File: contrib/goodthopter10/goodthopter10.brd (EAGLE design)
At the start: 210.2 x 143.8 mm, 24 parts, among them IC1 F22X4---DA38, IC2 FT232RL-BASICSSOP, Q2 20MHz

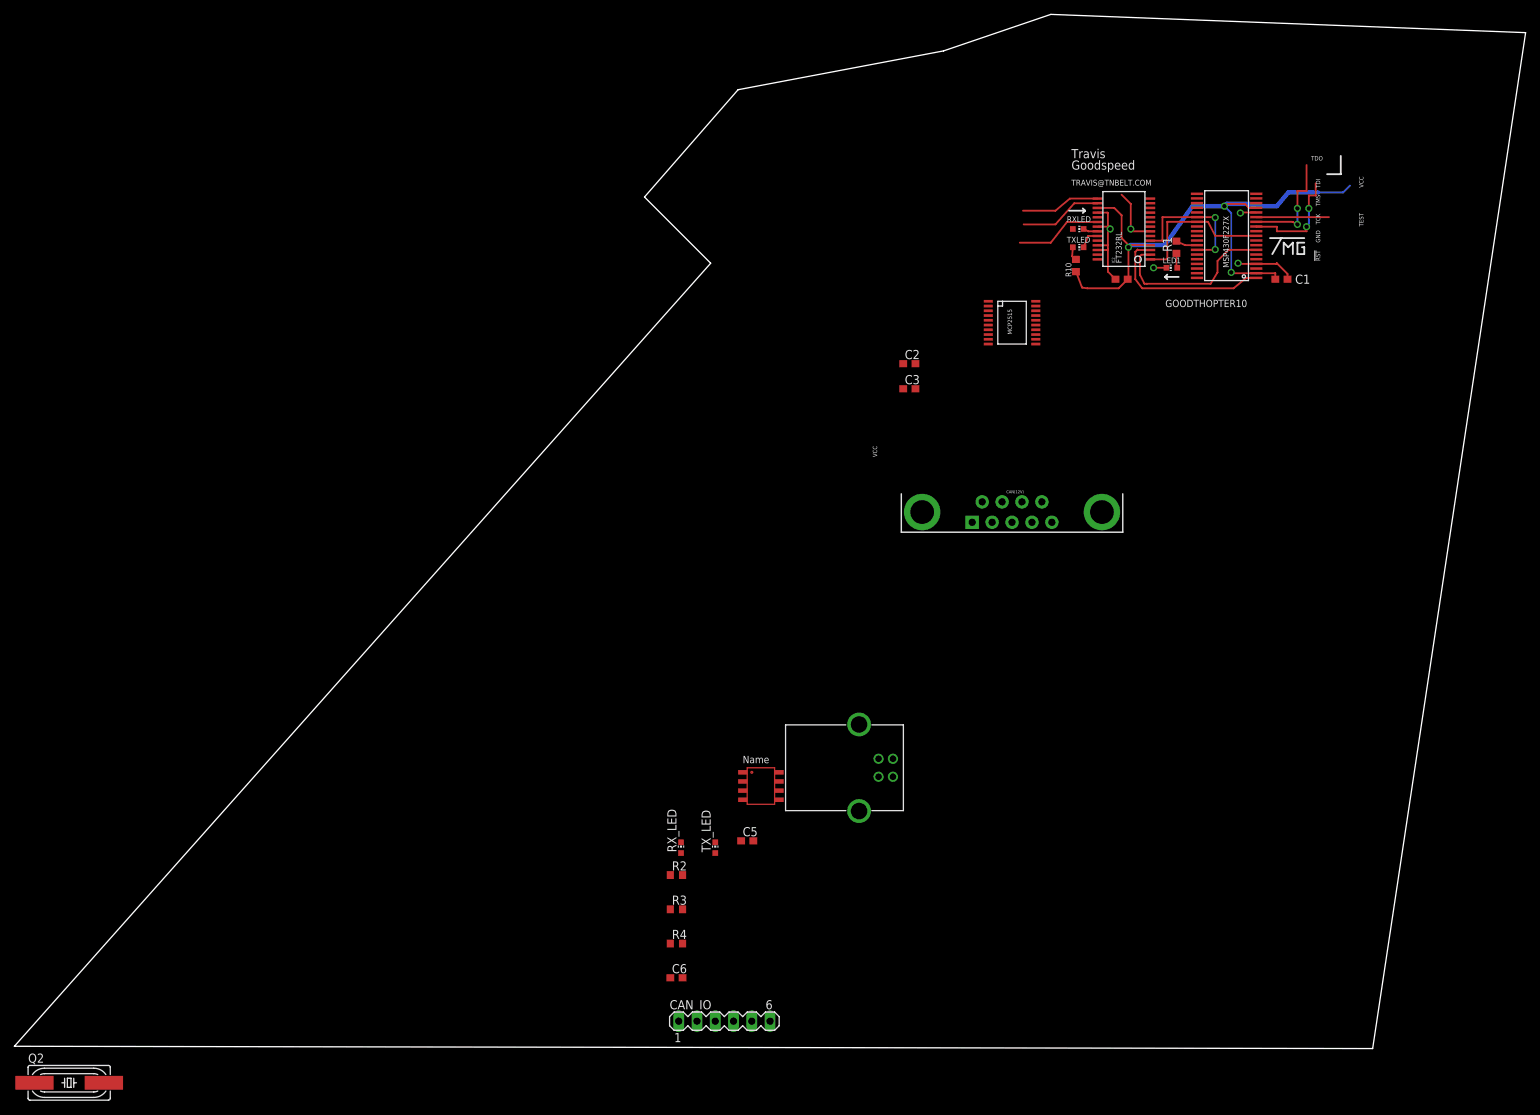
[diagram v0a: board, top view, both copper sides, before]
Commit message: Routing goodthopter10.brd, updated.
git-svn-id: https://svn.code.sf.net/p/goodfet/code@1213 12e2690d-a6be-4b82-a7b7-67c4a43b65c8
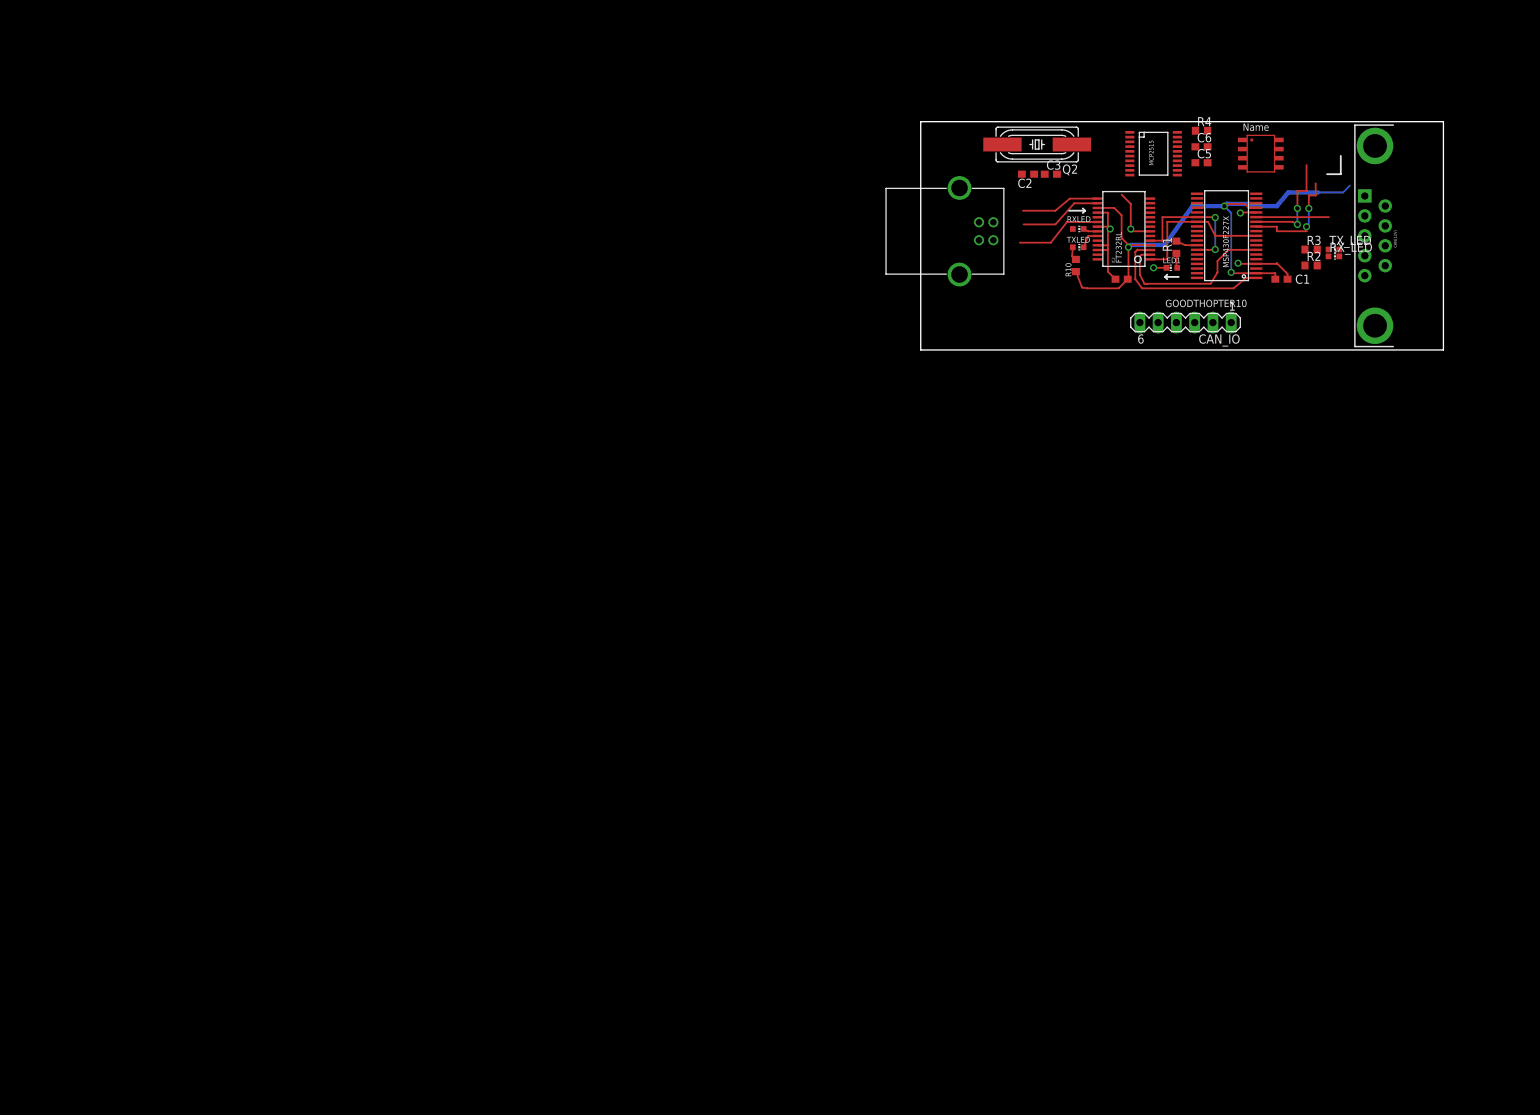
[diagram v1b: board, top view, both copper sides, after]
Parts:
- moved Q2 187.5 mm to (7.62, 21.6), turned to 180 degrees
- moved C6 136.7 mm to (30.5, 21.3)
- moved R4 134.6 mm to (30.5, 23.5)
- moved R3 127.3 mm to (45.7, 6.99)
- moved RX_LED 122.5 mm to (48.9, 6.03), turned to 270 degrees
- moved R2 122.4 mm to (45.7, 4.76)
- moved TX_LED 119.7 mm to (48.9, 6.99), turned to 270 degrees
- moved CAN_IO 116.4 mm to (28.3, -3.17), turned to 180 degrees
- moved C5 113.5 mm to (30.5, 19.1)
- moved U$2 112.1 mm to (38.7, 20.3)
- moved 292304-2 75.9 mm to (-3.17, 9.53)
- moved CAN(12V) 63.4 mm to (54.6, 8.89), turned to 270 degrees
- moved C3 35.8 mm to (9.53, 17.5)
- moved C2 31.1 mm to (6.35, 17.5), turned to 180 degrees
- moved U$1 30.7 mm to (23.8, 20.6)
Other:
- board size 210.2 x 143.8 mm -> 72.7 x 31.8 mm
- board text removed: "!RST"
- board text removed: "GND"
- board text removed: "Goodspeed"
- board text removed: "TCK"
- board text removed: "TDI"
- board text removed: "TDO"
- board text removed: "TEST"
- board text removed: "TMS"
- board text removed: "TRAVIS@TNBELT.COM"
- board text removed: "Travis"
- board text removed: "VCC"

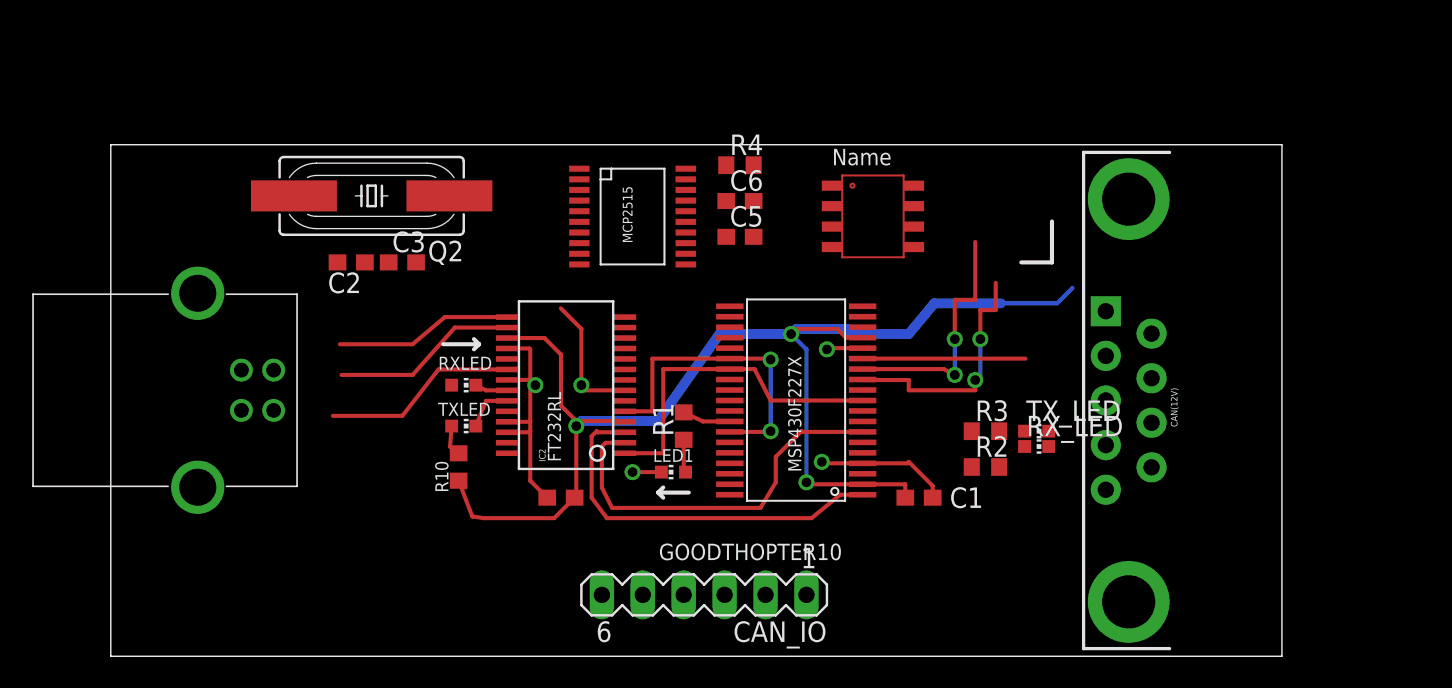
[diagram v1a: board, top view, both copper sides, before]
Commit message: Completed GoodThopter10 Routing, Gerbers Added, README.
git-svn-id: https://svn.code.sf.net/p/goodfet/code@1214 12e2690d-a6be-4b82-a7b7-67c4a43b65c8
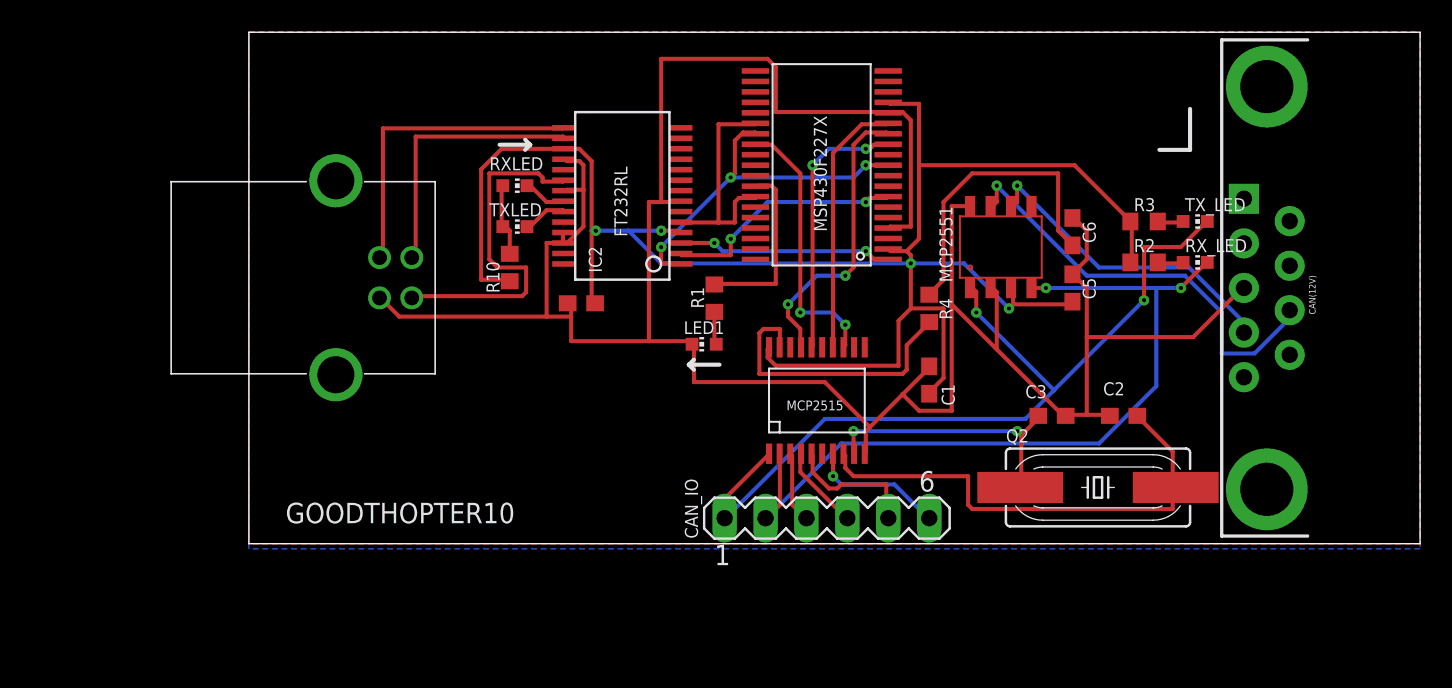
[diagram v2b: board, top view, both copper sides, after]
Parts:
- moved C2 48.9 mm to (54.3, 7.94), turned to 0 degrees
- moved Q2 48.6 mm to (52.7, 3.49), turned to 0 degrees
- moved C3 41.4 mm to (49.8, 7.94), turned to 180 degrees
- moved C5 20.9 mm to (51.1, 15.9), turned to 270 degrees
- moved C6 20.7 mm to (51.1, 19.4), turned to 270 degrees
- moved R3 16.3 mm to (55.6, 20.0)
- moved TX_LED 16.3 mm to (58.7, 20.0)
- moved U$1 16.2 mm to (34.9, 8.89), turned to 90 degrees
- moved R2 16.1 mm to (55.6, 17.5)
- moved RX_LED 15.1 mm to (58.7, 17.5)
- moved R4 14.7 mm to (42.2, 14.6), turned to 270 degrees
- moved IC1 14.7 mm to (35.6, 23.5)
- moved RXLED 12.8 mm to (16.5, 22.2)
- moved R10 12.8 mm to (16.2, 17.1)
- moved TXLED 12.8 mm to (16.5, 19.7)
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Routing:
- net GND: track 38.1 -> 163.2 mm, vias 5 -> 0
- net TXCAN: track 0.00 -> 53.2 mm, vias 0 -> 2
- net RXCAN: track 0.00 -> 49.7 mm, vias 0 -> 2
- net VCC: track 82.7 -> 115.8 mm, vias 3 -> 4
- net OSC2: track 0.00 -> 30.2 mm
- net CANH: track 0.00 -> 26.9 mm, vias 0 -> 1
- net CANL: track 0.00 -> 19.7 mm, vias 0 -> 1
- net N$11: track 0.00 -> 18.8 mm
- net N$5: track 0.00 -> 17.8 mm
- net OSC1: track 0.00 -> 16.8 mm, vias 0 -> 2
- net !INT: track 0.00 -> 16.7 mm, vias 0 -> 2
- net RTS: track 24.0 -> 13.3 mm, vias 0 -> 2
- net VCC5V: track 12.2 -> 21.6 mm
- net DTR: track 24.2 -> 15.0 mm, vias 0 -> 2
- net !TX2RTS: track 0.00 -> 8.43 mm, vias 0 -> 1
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- added copper zone on layer 1, net GND
- added copper zone on layer 16, net GND
